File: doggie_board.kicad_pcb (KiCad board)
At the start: 2 copper layers, 128 x 129 mm, 70 parts, among them J1 XT90PW-M, J5V1 Conn_01x02, J5V10 Conn_01x02, J5V11 Conn_01x02, J5V12 Conn_01x02, J5V13 Conn_01x02, J5V14 Conn_01x02, J5V15 Conn_01x02, J5V16 Conn_01x02, J5V17 Conn_01x02, J5V18 Conn_01x02, J5V19 Conn_01x02, J5V2 Conn_01x02, J5V20 Conn_01x02, J5V3 Conn_01x02, J5V4 Conn_01x02, J5V5 Conn_01x02, J5V6 Conn_01x02, J5V7 Conn_01x02, J5V8 Conn_01x02, J5V9 Conn_01x02, Q1 PSMN3R7-100BSEJ, Q2 PSMN3R7-100BSEJ, Q3 PSMN3R7-100BSEJ, Q4 PSMN3R7-100BSEJ, Q5 PSMN3R7-100BSEJ, U1 TPS2490, U2 LM76005, U3 LM76005, U4 LM76005

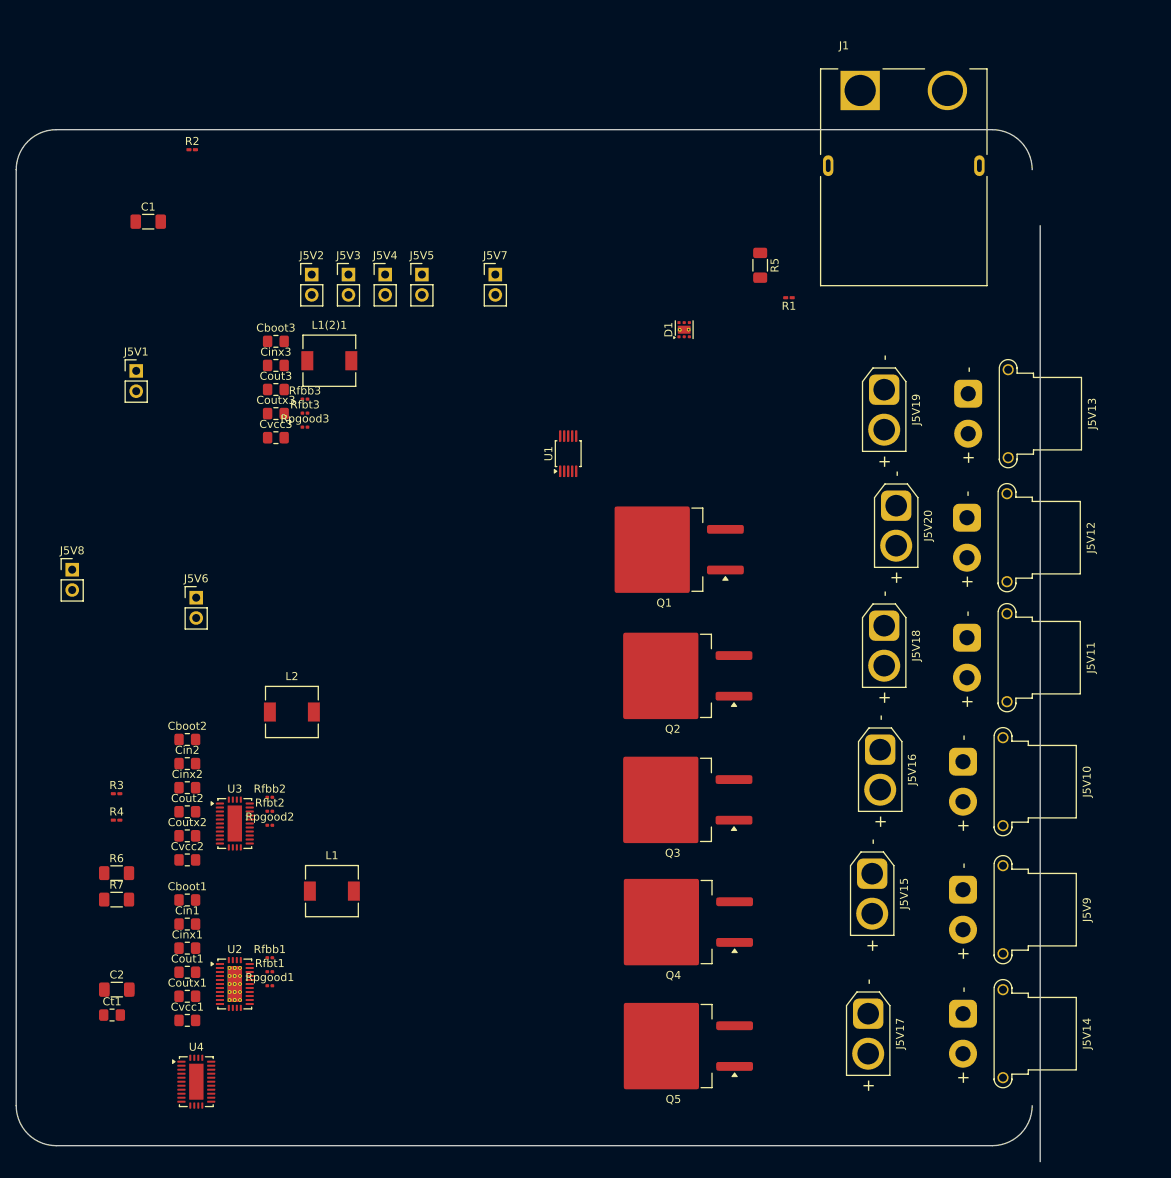
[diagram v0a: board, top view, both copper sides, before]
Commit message: updates
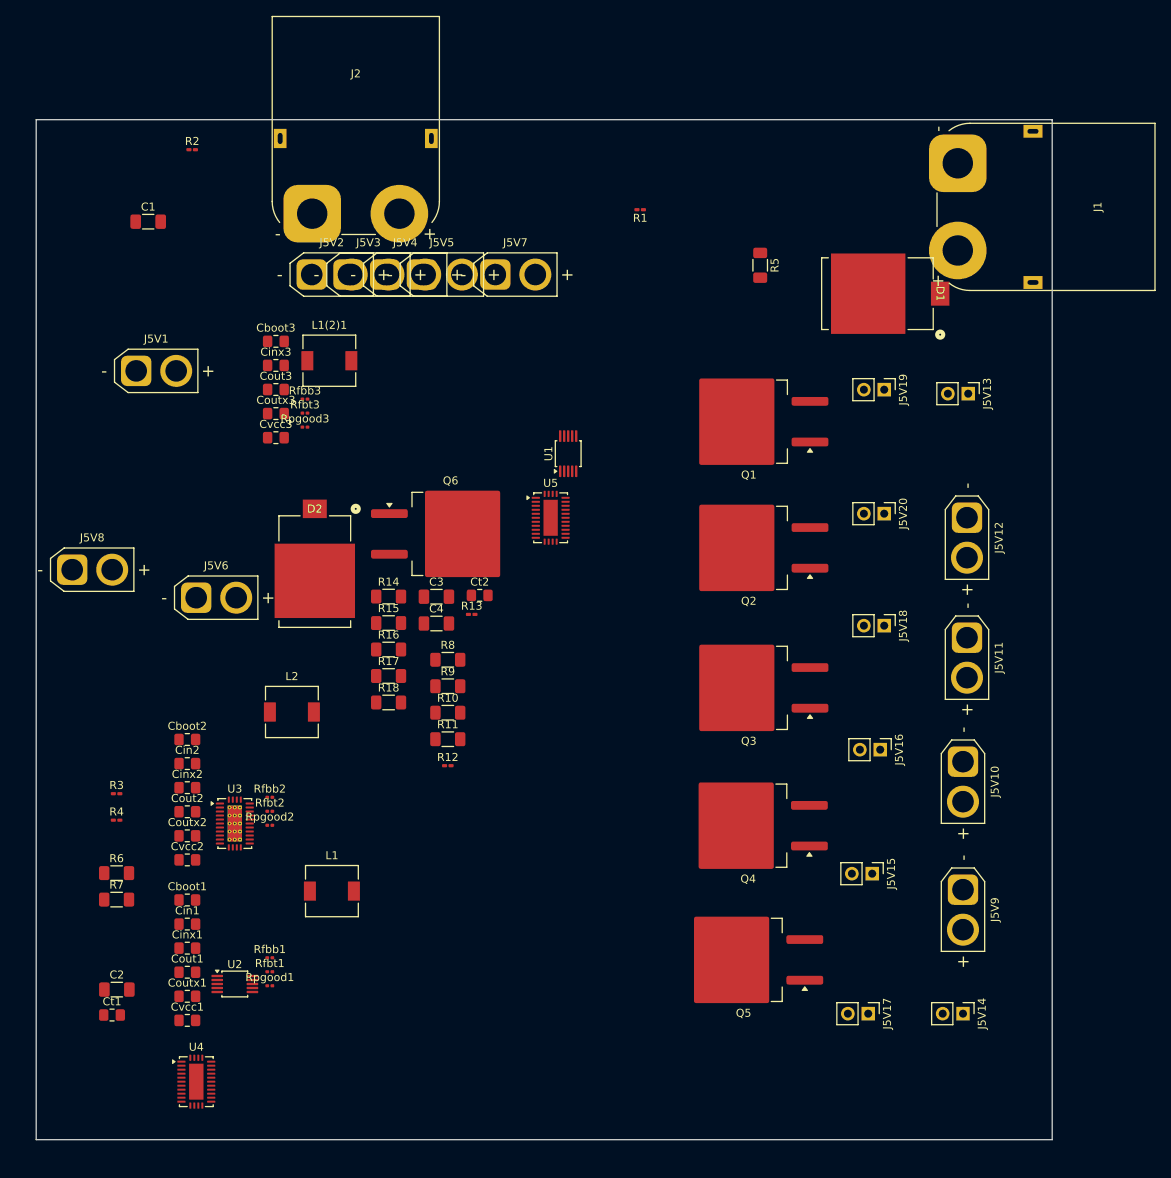
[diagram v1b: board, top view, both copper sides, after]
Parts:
- added C3: 0.1uF, 100V, Capacitor_SMD:C_1206_3216Metric_Pad1.33x1.80mm_HandSolder, F.Cu at (79.0, 98.9)
- added C4: 27nF, 100V, Capacitor_SMD:C_1206_3216Metric_Pad1.33x1.80mm_HandSolder, F.Cu at (79.0, 102.2)
- added Ct2: 1nF, Capacitor_SMD:C_0805_2012Metric_Pad1.18x1.45mm_HandSolder, F.Cu at (84.4, 98.7)
- added D2: 15KPA048C-SD-Q, footprints:DIODE_15KPA048C-SD-Q_BRN, F.Cu at (63.8, 95.7)
- added J2: XT90PW-M, Connector_AMASS:AMASS_XT90PW-M_1x02_P10.90mm_Horizontal, F.Cu at (63.5, 51.0)
- added Q6: PSMN3R7-100BSEJ, Package_TO_SOT_SMD:TO-263-2, F.Cu at (80.8, 91.0)
- added R10: 50, Resistor_SMD:R_1206_3216Metric_Pad1.30x1.75mm_HandSolder, F.Cu at (80.5, 113.4)
- added R11: 50, Resistor_SMD:R_1206_3216Metric_Pad1.30x1.75mm_HandSolder, F.Cu at (80.5, 116.7)
- added R12: 100k, Resistor_SMD:R_0201_0603Metric_Pad0.64x0.40mm_HandSolder, F.Cu at (80.5, 120.0)
- added R13: 18k, Resistor_SMD:R_0201_0603Metric_Pad0.64x0.40mm_HandSolder, F.Cu at (83.4, 101.1)
- added R14: 0.2m, 15W, Resistor_SMD:R_1206_3216Metric_Pad1.30x1.75mm_HandSolder, F.Cu at (73.0, 98.9)
- added R15: 50, Resistor_SMD:R_1206_3216Metric_Pad1.30x1.75mm_HandSolder, F.Cu at (73.0, 102.2)
- added R16: 50, Resistor_SMD:R_1206_3216Metric_Pad1.30x1.75mm_HandSolder, F.Cu at (73.0, 105.5)
- added R17: 50, Resistor_SMD:R_1206_3216Metric_Pad1.30x1.75mm_HandSolder, F.Cu at (73.0, 108.8)
- added R18: 1k, Resistor_SMD:R_1206_3216Metric_Pad1.30x1.75mm_HandSolder, F.Cu at (73.0, 112.1)
- added R8: 50, Resistor_SMD:R_1206_3216Metric_Pad1.30x1.75mm_HandSolder, F.Cu at (80.5, 106.8)
- added R9: 1k, Resistor_SMD:R_1206_3216Metric_Pad1.30x1.75mm_HandSolder, F.Cu at (80.5, 110.1)
- added U5: LM76005, Package_DFN_QFN:Texas_RNP0030B_WQFN-30-1EP_4x6mm_P0.5mm_EP1.8x4.5mm, F.Cu at (93.3, 89.0)
- D1: value SMF48A -> 15KPA048C-SD-Q; footprint Package_SON:WSON-6-1EP_2x2mm_P0.65mm_EP1x1.6mm_ThermalVias -> footprints:DIODE_15KPA048C-SD-Q_BRN
- J1: footprint vssop:AMASS_XT90PW-M -> Connector_AMASS:AMASS_XT90PW-M_1x02_P10.90mm_Horizontal
- J5V1, J5V2, J5V3, J5V4, J5V5, J5V6, J5V7, J5V8: footprint Connector_PinHeader_2.54mm:PinHeader_1x02_P2.54mm_Vertical -> Connector_AMASS:AMASS_XT30U-F_1x02_P5.0mm_Vertical
- J5V10, J5V11, J5V12, J5V9: footprint Connector_AMASS:AMASS_XT30PW-F_1x02_P2.50mm_Horizontal -> Connector_AMASS:AMASS_XT30U-F_1x02_P5.0mm_Vertical
- J5V13, J5V14: footprint Connector_AMASS:AMASS_XT30PW-F_1x02_P2.50mm_Horizontal -> Connector_PinHeader_2.54mm:PinHeader_1x02_P2.54mm_Vertical
- J5V15, J5V16, J5V17, J5V18, J5V19, J5V20: footprint Connector_AMASS:AMASS_XT30U-F_1x02_P5.0mm_Vertical -> Connector_PinHeader_2.54mm:PinHeader_1x02_P2.54mm_Vertical
- R6: value 10 -> 50
- R7: value 1k -> 50
- U2: value LM76005 -> TPS2490; footprint Package_DFN_QFN:Texas_RNP0030B_WQFN-30-1EP_4x6mm_P0.5mm_EP1.8x4.5mm_ThermalVias -> Package_SO:VSSOP-10_3x3mm_P0.5mm
- U3: footprint Package_DFN_QFN:Texas_RNP0030B_WQFN-30-1EP_4x6mm_P0.5mm_EP1.8x4.5mm -> Package_DFN_QFN:Texas_RNP0030B_WQFN-30-1EP_4x6mm_P0.5mm_EP1.8x4.5mm_ThermalVias
- moved D1 24.6 mm to (134.2, 61.0), turned to -90 degrees
- moved R1 21.6 mm to (104.5, 50.5)
- moved Q1 19.2 mm to (118.1, 77.0)
- moved Q2 18.6 mm to (118.1, 92.8)
- moved Q3 16.9 mm to (118.1, 110.3)
- moved Q4 15.3 mm to (118.0, 127.5)
- moved Q5 13.9 mm to (117.4, 144.3)
- moved J1 6.76 mm to (144.2, 44.7), turned to -90 degrees
- moved J5V20 1.80 mm to (135.0, 88.5)
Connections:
- net /High Side Power Switch/SWITCH_HIGH renamed Net-(SW1-A)
- C1 pad 1: +48V -> 48_L
- Cboot1 pad 1: Net-(U2-BOOT) -> Net-(U3-BOOT)
- Cboot2 pad 1: Net-(U3-BOOT) -> Net-(U4-BOOT)
- Cboot3 pad 1: Net-(U4-BOOT) -> Net-(U5-BOOT)
- Cvcc1 pad 1: Net-(U2-VCC) -> Net-(U3-VCC)
- Cvcc2 pad 1: Net-(U3-VCC) -> Net-(U4-VCC)
- Cvcc3 pad 1: Net-(U4-VCC) -> Net-(U5-VCC)
- D1 pad 1: +48V -> 48_L
- J5V1 pad 1: +5V -> 48v_switched
- J5V10 pad 1: +48V -> 48v_switched
- J5V11 pad 1: +48V -> 48v_switched
- J5V12 pad 1: +48V -> 48v_switched
- J5V13 pad 1: +48V -> +3.3V
- J5V14 pad 1: +48V -> +3.3V
- J5V15 pad 1: +48V -> +3.3V
- J5V16 pad 1: +48V -> +3.3V
- J5V17 pad 1: +48V -> +5V
- J5V18 pad 1: +48V -> +5V
- J5V19 pad 1: +48V -> +5V
- J5V2 pad 1: +5V -> 48v_switched
- J5V20 pad 1: +48V -> +5V
- J5V3 pad 1: +5V -> 48v_switched
- J5V4 pad 1: +5V -> 48v_switched
- J5V5 pad 1: +3.3V -> 48v_switched
- J5V6 pad 1: +3.3V -> 48v_switched
- J5V7 pad 1: +3.3V -> 48v_switched
- J5V8 pad 1: +3.3V -> 48v_switched
- J5V9 pad 1: +48V -> 48v_switched
- Q1 pad 1: /High Side Power Switch/gate_line -> Net-(Q1-Pad1)
- Q1 pad 3: 48v_switched -> +48V
- Q2 pad 1: /High Side Power Switch/gate_line -> Net-(Q2-Pad1)
- Q2 pad 3: 48v_switched -> +48V
- Q3 pad 1: /High Side Power Switch/gate_line -> Net-(Q3-Pad1)
- Q3 pad 3: 48v_switched -> +48V
- Q4 pad 1: /High Side Power Switch/gate_line -> Net-(Q4-Pad1)
- Q4 pad 3: 48v_switched -> +48V
- Q5 pad 1: /High Side Power Switch/gate_line -> Net-(Q5-Pad1)
- Q5 pad 3: 48v_switched -> +48V
- R1 pad 1: +48V -> 48_L
- R5 pad 1: +48V -> 48_L
- R6 pad 1: Net-(U1-GATE) -> /High Side Power Switch/gate_line
- R6 pad 2: /High Side Power Switch/gate_line -> Net-(Q1-Pad1)
- R7 pad 2: Net-(C2-Pad1) -> Net-(Q2-Pad1)
- Rfbb1 pad 1: Net-(U2-FB) -> Net-(U3-FB)
- Rfbb2 pad 1: Net-(U3-FB) -> Net-(U4-FB)
- Rfbb3 pad 1: Net-(U4-FB) -> Net-(U5-FB)
- Rfbt1 pad 2: Net-(U2-FB) -> Net-(U3-FB)
- Rfbt2 pad 2: Net-(U3-FB) -> Net-(U4-FB)
- Rfbt3 pad 2: Net-(U4-FB) -> Net-(U5-FB)
- Rpgood1 pad 1: Net-(U2-PGOOD) -> Net-(U3-PGOOD)
- Rpgood2 pad 1: Net-(U3-PGOOD) -> Net-(U4-PGOOD)
- Rpgood3 pad 2: Net-(U4-PGOOD) -> Net-(U5-PGOOD)
- U1 pad 1: Net-(SW1-B) -> ps_sw
- U1 pad 10: +48V -> 48_L
- U1 pad 7: 48v_switched -> +48V
- U1 pad 8: Net-(U1-GATE) -> /High Side Power Switch/gate_line
- U2 pad 1: Net-(Cboot1-Pad2) -> ps_sw
- U2 pad 10: unconnected-(U2-RT-Pad10) -> 48_R
- U2 pad 2: Net-(Cboot1-Pad2) -> Net-(U2-VREF)
- U2 pad 3: Net-(Cboot1-Pad2) -> Net-(U2-PROG)
- U2 pad 4: Net-(Cboot1-Pad2) -> Net-(U2-TIMER)
- U2 pad 5: Net-(Cboot1-Pad2) -> GND
- U2 pad 6: Net-(U2-BOOT) -> unconnected-(U2-PG-Pad6)
- U2 pad 7: unconnected-(U2-NC-Pad7) -> +48V
- U2 pad 8: Net-(U2-VCC) -> /High Side Power Switch/gate_line
- U2 pad 9: GND -> /High Side Power Switch/drain
- U3 pad 1: Net-(Cboot2-Pad2) -> Net-(Cboot1-Pad2)
- U3 pad 10: GND -> unconnected-(U3-RT-Pad10)
- U3 pad 11: GND -> unconnected-(U3-SS/TRK-Pad11)
- U3 pad 2: Net-(Cboot2-Pad2) -> Net-(Cboot1-Pad2)
- U3 pad 3: Net-(Cboot2-Pad2) -> Net-(Cboot1-Pad2)
- U3 pad 4: Net-(Cboot2-Pad2) -> Net-(Cboot1-Pad2)
- U3 pad 5: Net-(Cboot2-Pad2) -> Net-(Cboot1-Pad2)
- U4 pad 1: Net-(Cboot3-Pad2) -> Net-(Cboot2-Pad2)
- U4 pad 10: unconnected-(U4-RT-Pad10) -> GND
- U4 pad 11: unconnected-(U4-SS/TRK-Pad11) -> GND
- U4 pad 2: Net-(Cboot3-Pad2) -> Net-(Cboot2-Pad2)
- U4 pad 3: Net-(Cboot3-Pad2) -> Net-(Cboot2-Pad2)
- U4 pad 4: Net-(Cboot3-Pad2) -> Net-(Cboot2-Pad2)
- U4 pad 5: Net-(Cboot3-Pad2) -> Net-(Cboot2-Pad2)
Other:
- board size 128 x 129 mm -> 127 x 127.5 mm
